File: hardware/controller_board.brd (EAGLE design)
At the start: 86 x 71.5 mm, 95 parts, among them J1 USB-MICROA-AMPHENOL-10118192-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, J2 2.4K, J3 2.4K, J4 AVR_SPI_PRG_6-SMD, J7 FRSKY-GIMBAL-2X-SERVO-SMD, J8 FRSKY-GIMBAL-2X-SERVO-SMD, P1 TEST-POINT, P2 TEST-POINT, P3 TEST-POINT, P4 TEST-POINT, U2 MCP73831T-2ACI/OT, U3 FT232RLSSOP, U4 ATMEGA128RFA1, U5 DPDT-X2, Y1 CRYSTAL5X3

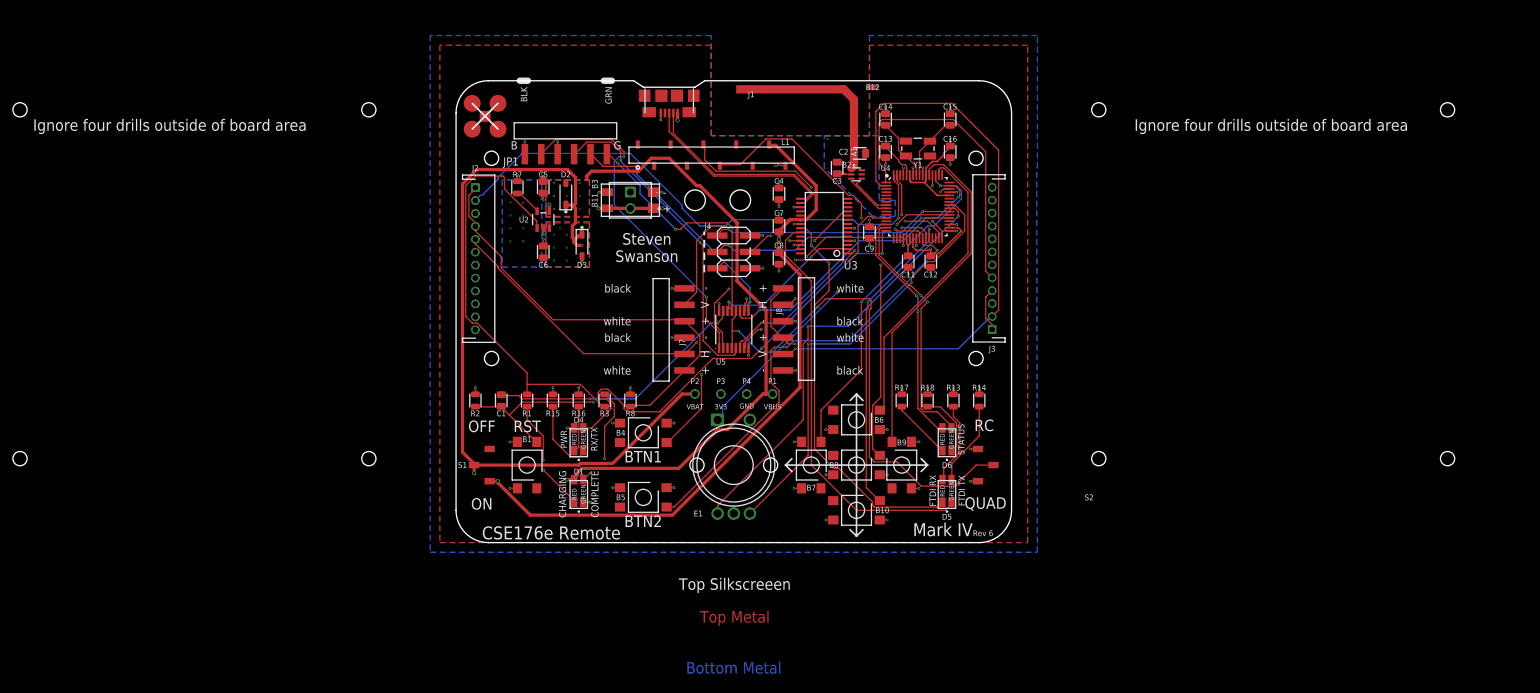
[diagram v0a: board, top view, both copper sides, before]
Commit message: passes eaglint.
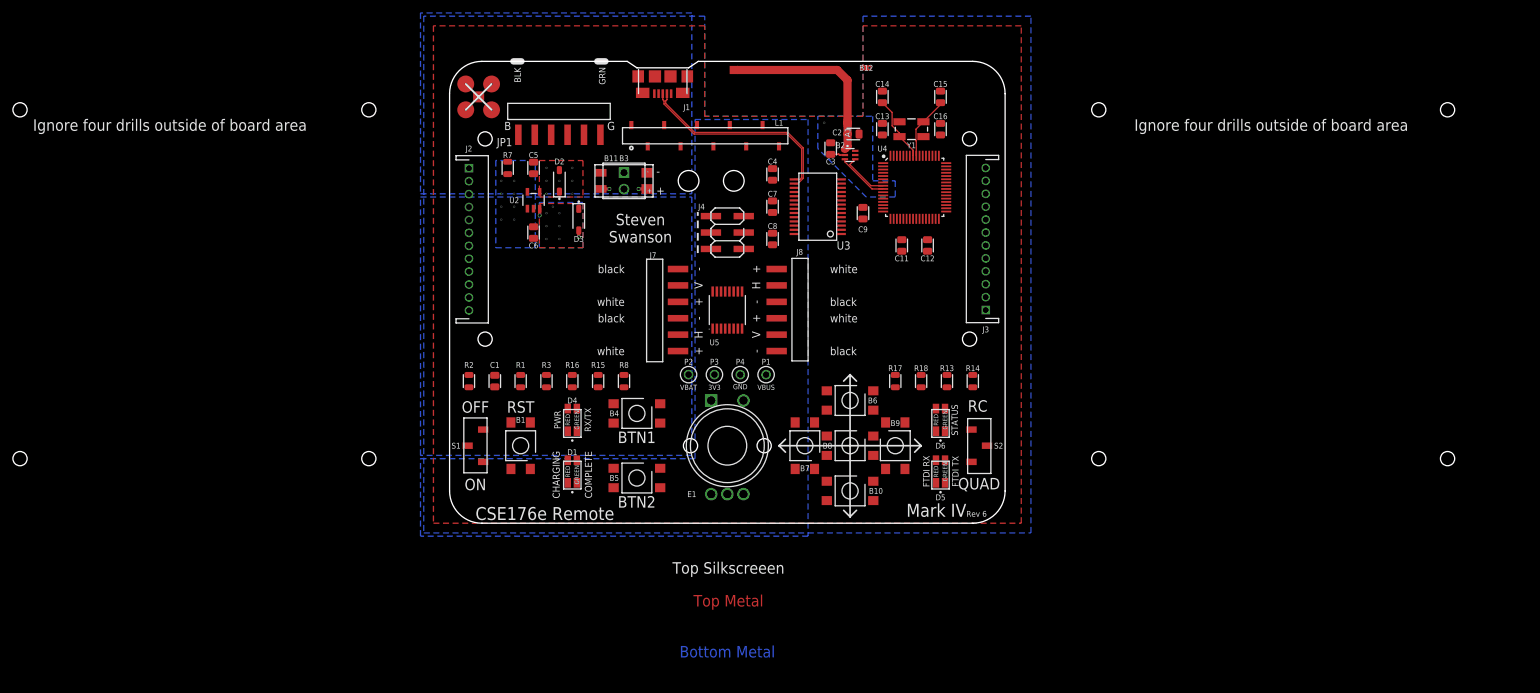
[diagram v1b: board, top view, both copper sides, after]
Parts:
- removed V10: LOCKED-VIA-0.2, quadparts_prebuilt:VIA-0.2MM
- moved U$4 29.2 mm to (-72.0, 2.00)
- moved R3 9.49 mm to (-29.0, -15.0)
- moved R15 7.62 mm to (-21.0, -15.0)
- moved D3 4.03 mm to (-24.0, 10.0)
- moved C15 3.81 mm to (32.0, 29.0)
- moved C16 3.81 mm to (32.0, 24.0)
- moved V3 3.63 mm to (-36.0, 16.0)
- moved V35 3.63 mm to (-34.0, 12.0)
- moved V37 3.63 mm to (-34.0, 14.0)
- moved V38 3.63 mm to (-36.0, 12.0)
- moved V4 3.63 mm to (-36.0, 10.0)
- moved V5 3.63 mm to (-34.0, 10.0)
- moved V7 3.63 mm to (-36.0, 14.0)
- moved V8 3.63 mm to (-34.0, 16.0)
- moved V30 3.54 mm to (-27.0, 9.00)
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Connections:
- removed net BAT_SENSE: U4.3
- net VBAT: no longer V10.P1
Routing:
- net GREF: track 133.2 -> 0.00 mm, vias 2 -> 0
- net VBAT: track 120.4 -> 0.00 mm, vias 3 -> 0
- net VBUS: track 117.8 -> 0.00 mm, vias 4 -> 0
- net VREG_IN: track 104.9 -> 0.00 mm, vias 3 -> 0
- net THROTTLE: track 97.9 -> 0.00 mm, vias 2 -> 0
- net PITCH: track 96.1 -> 0.00 mm, vias 1 -> 0
- net YAW: track 91.9 -> 0.00 mm, vias 2 -> 0
- net RESET: track 88.5 -> 0.00 mm, vias 3 -> 0
- net ROLL: track 82.6 -> 0.00 mm, vias 1 -> 0
- net PROG_SEL: track 79.1 -> 0.00 mm, vias 2 -> 0
- net GND: track 74.5 -> 0.00 mm, vias 59 -> 0
- net RF: track 69.4 -> 0.00 mm, vias 2 -> 0
- net BTN2/SDA: track 68.5 -> 0.00 mm, vias 2 -> 0
- net E1-A: track 67.4 -> 0.00 mm, vias 2 -> 0
- net E1-B: track 67.4 -> 0.00 mm, vias 2 -> 0
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- added copper zone on layer 16, net VBAT
- added copper zone on layer 16, net VREG_IN
- removed copper zone on layer 16, net 3V3
